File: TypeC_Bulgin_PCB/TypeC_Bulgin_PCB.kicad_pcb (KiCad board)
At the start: 2 copper layers, 16.1 x 16.1 mm, 4 parts, among them J1 Conn_01x01_Female, J3 Conn_01x13, J4 Conn_01x13, J6 USB_C_Receptacle

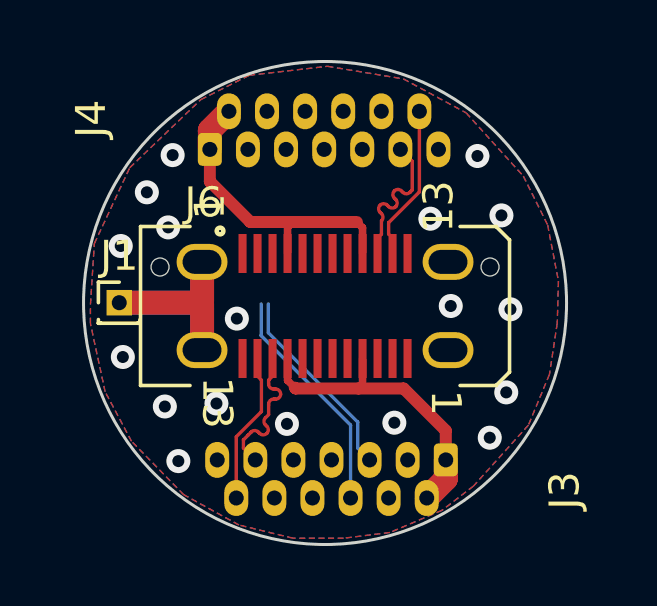
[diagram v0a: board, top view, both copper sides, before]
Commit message: v0.3 Seems 2B ready
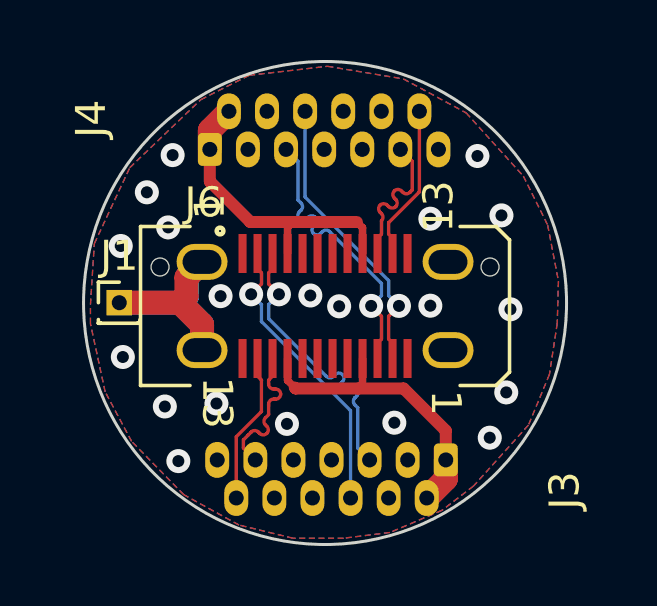
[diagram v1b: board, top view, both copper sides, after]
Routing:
- net TX2-: track 0.00 -> 9.73 mm, vias 0 -> 1
- net TX2+: track 0.00 -> 9.68 mm, vias 0 -> 1
- net TX1+: track 6.60 -> 9.67 mm, vias 0 -> 1
- net TX1-: track 7.70 -> 9.72 mm, vias 0 -> 1
- net GND: vias 18 -> 20
